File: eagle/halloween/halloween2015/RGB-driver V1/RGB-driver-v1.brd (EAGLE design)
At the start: 88.3 x 86.7 mm, 37 parts, among them IC1 MEGA8-AI, J1 RJ12RIGHTANGLE-I2C, J2 RJ12RIGHTANGLE-I2C, Q1 BSP75, Q10 BSP75, Q11 BSP75, Q12 BSP75, Q13 BSP75, Q14 BSP75, Q15 BSP75, Q16 BSP75, Q17 BSP75, Q18 BSP75, Q2 BSP75, Q3 BSP75, Q4 BSP75, Q5 BSP75, Q6 BSP75, Q7 BSP75, Q8 BSP75, Q9 BSP75

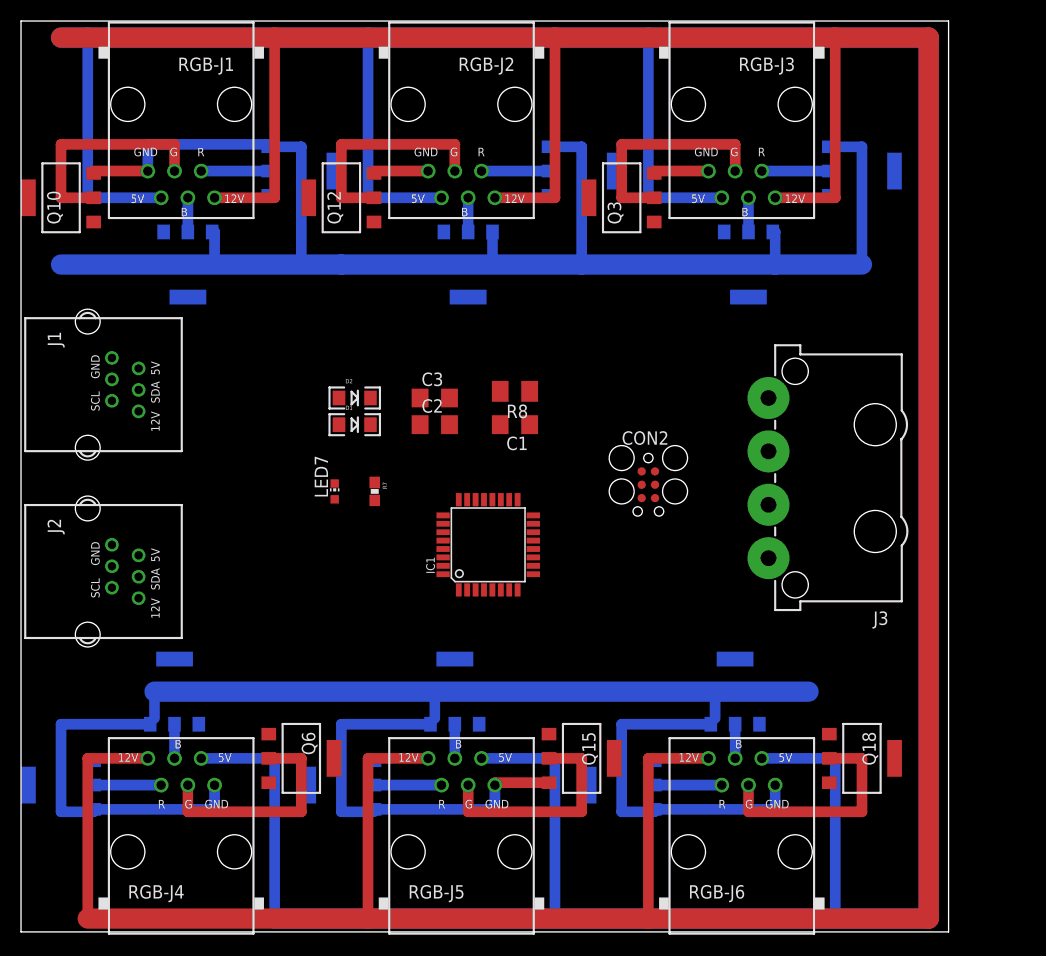
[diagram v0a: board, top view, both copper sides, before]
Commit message: Update libraries
t st# Please enter the commit message for your changes. Lines starting
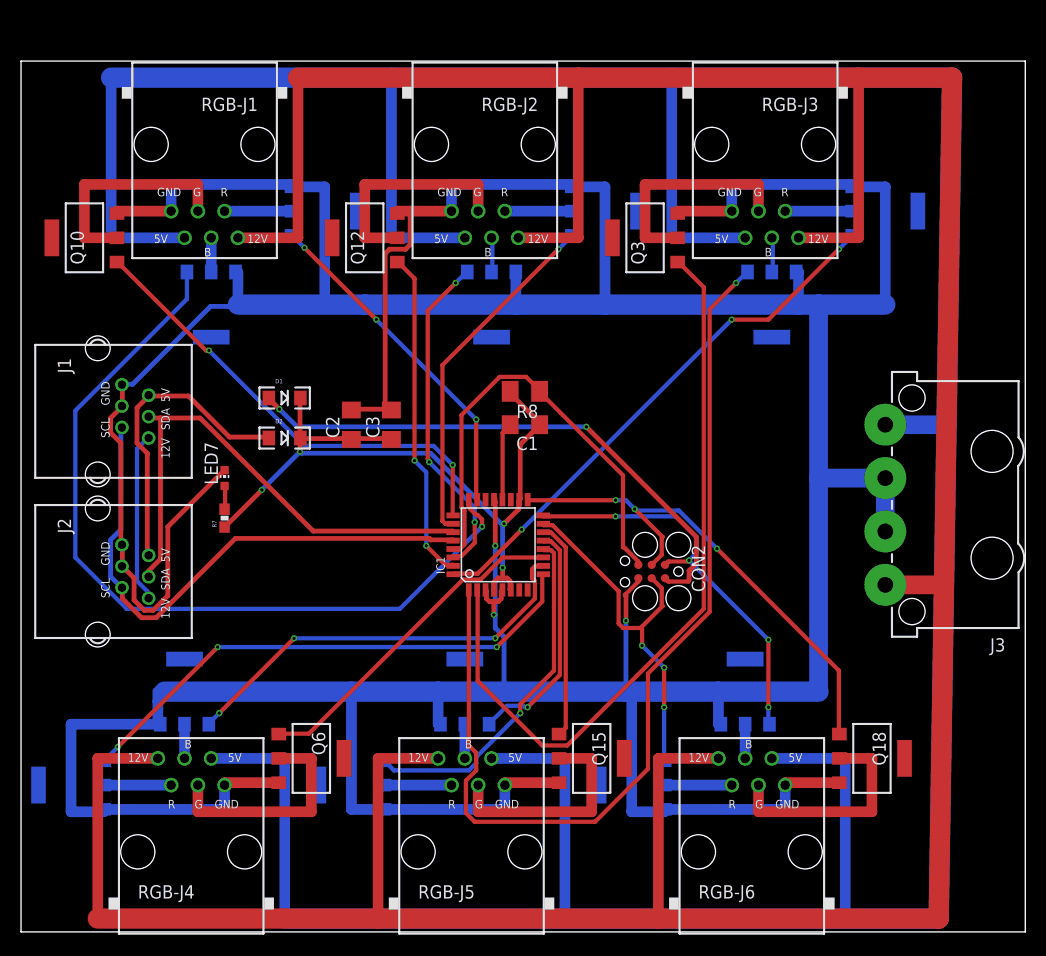
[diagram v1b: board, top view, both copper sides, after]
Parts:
- moved R7 14.5 mm to (19.4, 39.4), turned to 90 degrees
- moved J3 11.4 mm to (82.2, 40.6)
- moved CON2 11.2 mm to (62.5, 34.3), turned to 180 degrees
- moved LED7 10.6 mm to (19.4, 43.2)
- moved C2 7.94 mm to (31.4, 48.3), turned to 90 degrees
- moved D2 7.68 mm to (25.1, 47.0)
- moved D1 7.13 mm to (25.1, 50.8)
- moved C3 4.85 mm to (35.2, 48.3), turned to 90 degrees
- moved Q9 4.41 mm to (18.1, 59.7)
- moved Q1 4.41 mm to (82.2, 68.6)
- moved Q11 4.41 mm to (44.8, 59.7)
- moved Q2 4.41 mm to (71.4, 59.7)
- moved Q7 4.41 mm to (55.6, 68.6)
- moved Q8 4.41 mm to (28.9, 68.6)
- moved Q3 4.41 mm to (59.4, 66.0)
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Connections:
- net N$22 renamed GND
- net N$25 renamed +5V_HP
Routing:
- net GND: track 271.2 -> 530.3 mm, vias 0 -> 3
- net D3: track 0.00 -> 92.9 mm, vias 0 -> 1
- net A1: track 0.00 -> 78.7 mm, vias 0 -> 1
- net D4: track 0.00 -> 72.2 mm
- net +5V: track 0.00 -> 70.2 mm, vias 0 -> 4
- net N$18: track 64.8 -> 0.00 mm
- net 5V_A: track 0.00 -> 53.1 mm, vias 0 -> 2
- net SCL: track 0.00 -> 52.6 mm
- net D2: track 0.00 -> 51.4 mm, vias 0 -> 3
- net D5: track 0.00 -> 50.6 mm, vias 0 -> 3
- net SCK: track 0.00 -> 49.2 mm, vias 0 -> 3
- net SDA: track 0.00 -> 49.2 mm
- net A2: track 0.00 -> 44.7 mm, vias 0 -> 2
- net RESET: track 0.00 -> 43.6 mm
- net D6: track 0.00 -> 40.1 mm, vias 0 -> 3
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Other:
- board size 88.3 x 86.7 mm -> 95.6 x 82.9 mm
- board text added: "RGB High power V1"
